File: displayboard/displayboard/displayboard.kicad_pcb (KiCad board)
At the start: 2 copper layers, 105.3 x 56.3 mm, 8 parts

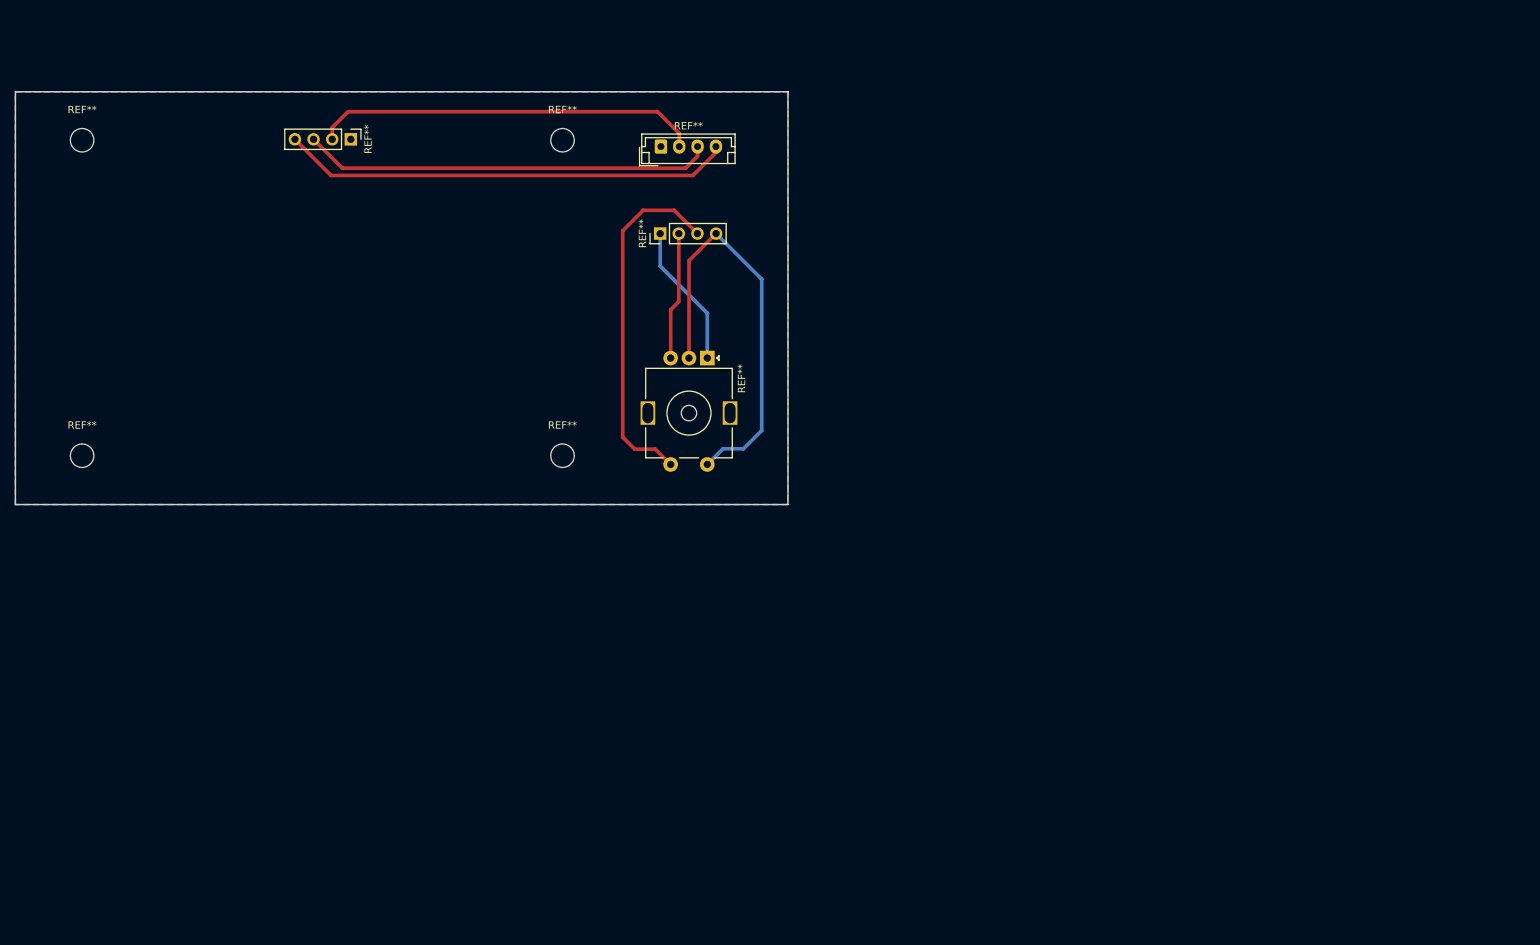
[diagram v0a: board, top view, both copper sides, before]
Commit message: V1.2
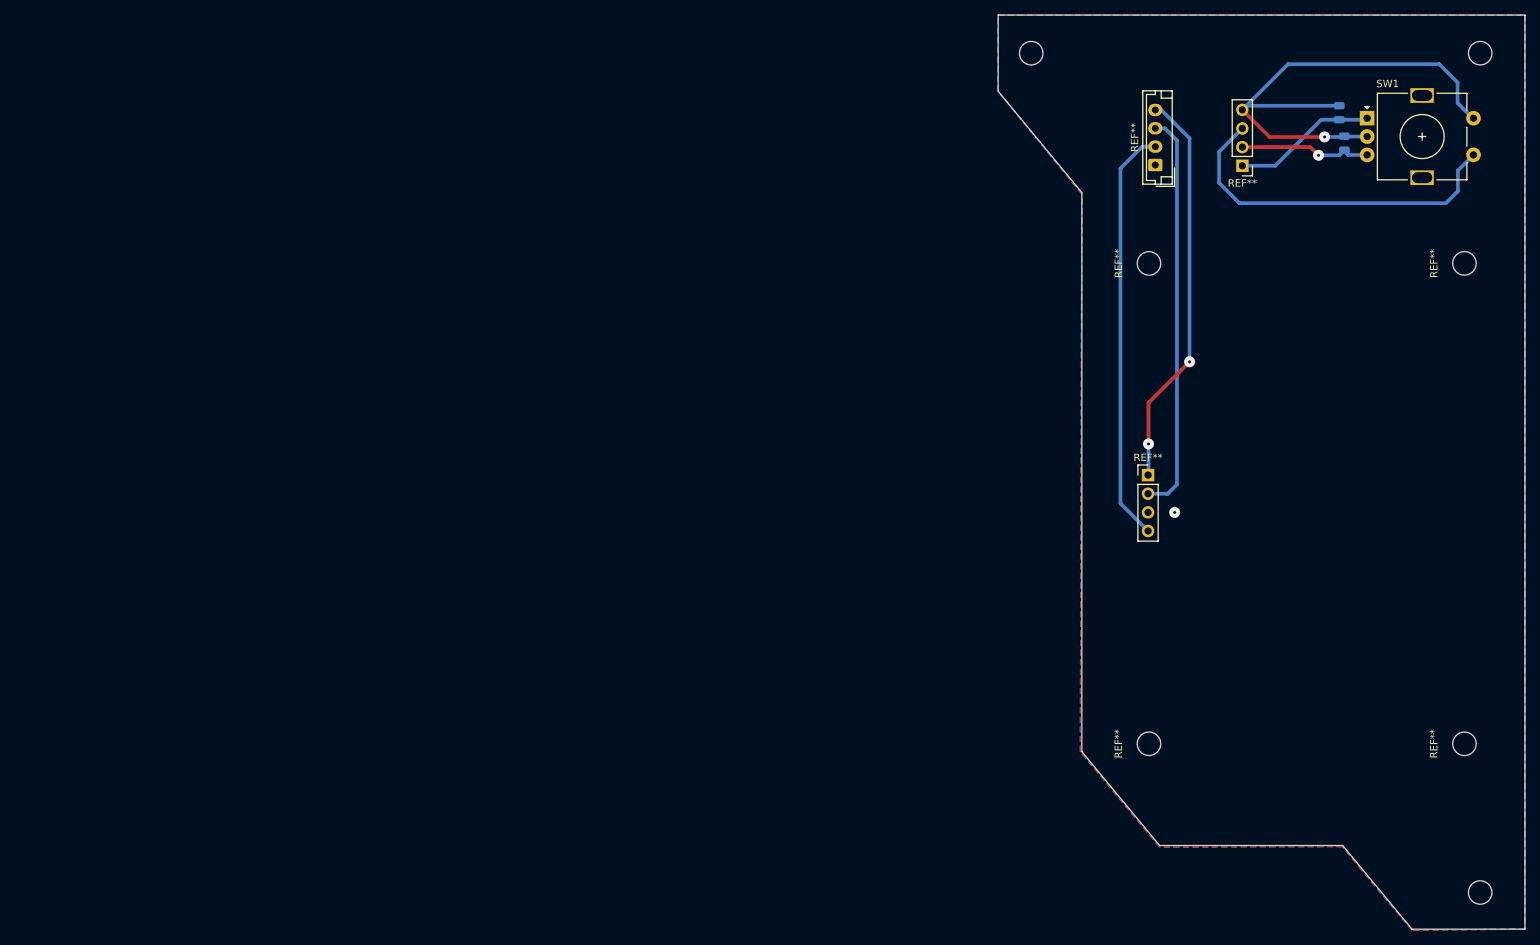
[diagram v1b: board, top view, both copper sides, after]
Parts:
- removed the REF** at (169.7, 68.8)
- added ?: , , F.Cu at (213.9, 27.2)
- added ?: , , F.Cu at (275.1, 27.2)
- added ?: , , F.Cu at (275.1, 141.6)
- added C1: C_Small, Capacitor_SMD:C_0805_2012Metric, B.Cu at (255.9, 35.3)
- added C2: C_Small, Capacitor_SMD:C_0805_2012Metric, B.Cu at (256.6, 39.5)
- added SW1: RotaryEncoder_Switch, Rotary_Encoder:RotaryEncoder_Alps_EC11E-Switch_Vertical_H20mm, F.Cu at (259.7, 36.1)
- moved REF** 192.5 mm to (273.0, 121.3), turned to 90 degrees
- moved REF** 167.1 mm to (230.0, 121.3), turned to 90 degrees
- moved REF** 125.7 mm to (273.0, 55.9), turned to 90 degrees
- moved REF** 117.9 mm to (229.8, 84.7), turned to 0 degrees
- moved REF** 81.7 mm to (230.0, 55.9), turned to 90 degrees
- moved REF** 79.9 mm to (242.7, 42.5), turned to 180 degrees
- moved REF** 67.4 mm to (230.8, 42.4), turned to 90 degrees
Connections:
- REF** pad 1: GND -> Net-(A1-GPIO20)
- REF** pad 2: PICO_3V3 -> Net-(A1-GPIO21)
- REF** pad 3: Net-(A1-GPIO21) -> GND
- REF** pad 4: Net-(A1-GPIO20) -> PICO_3V3
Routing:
- net AGND: track 57.3 -> 71.1 mm, vias 0 -> 1
- net Net-(A1-GPIO20): track 61.5 -> 54.5 mm, vias 0 -> 2
- net PICO_3V3: track 52.8 -> 57.0 mm
- net Net-(A1-GPIO21): track 56.0 -> 55.0 mm
- net ADC0_GP27: track 17.4 -> 18.0 mm, vias 0 -> 1
- net GND: vias 0 -> 1
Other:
- board size 105.3 x 56.3 mm -> 71.8 x 124.6 mm
